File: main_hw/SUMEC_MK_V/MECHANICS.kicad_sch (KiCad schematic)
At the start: 16 parts, among them SW2 SW_Push, SW3 SW_Push, SW4 SW_Push, SW5 SW_Push

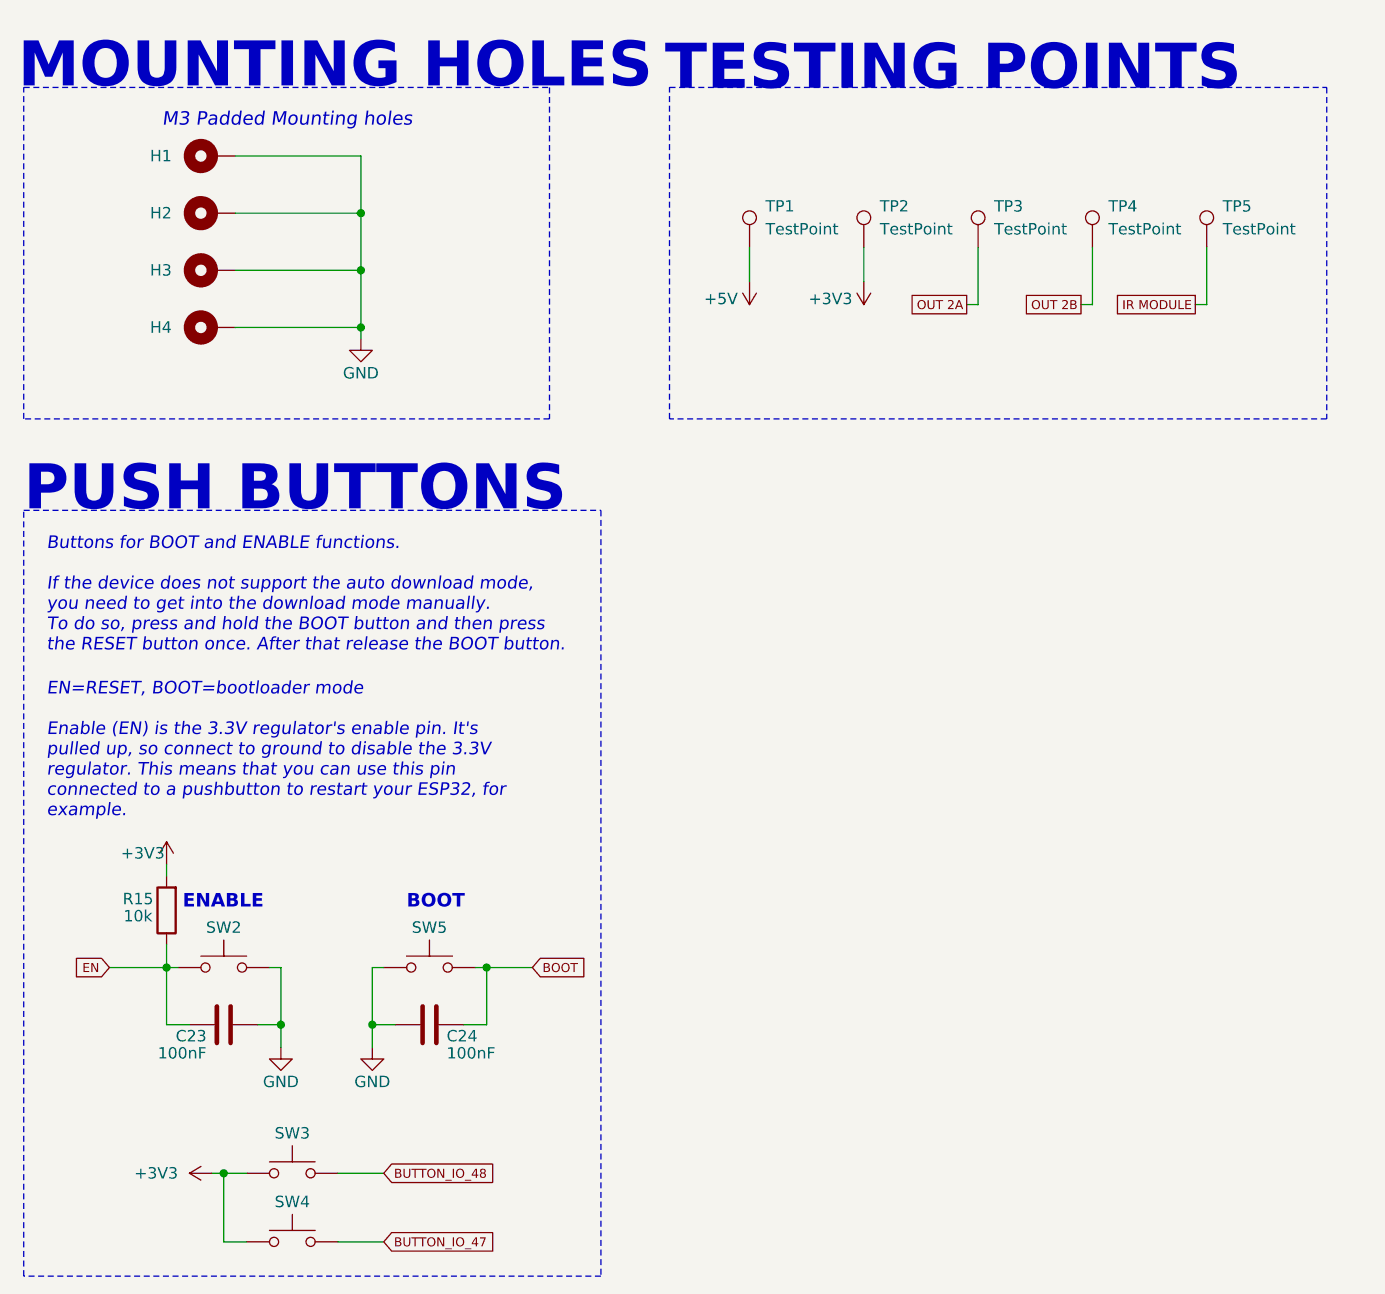
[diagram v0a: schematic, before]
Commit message: MK V Schematic update
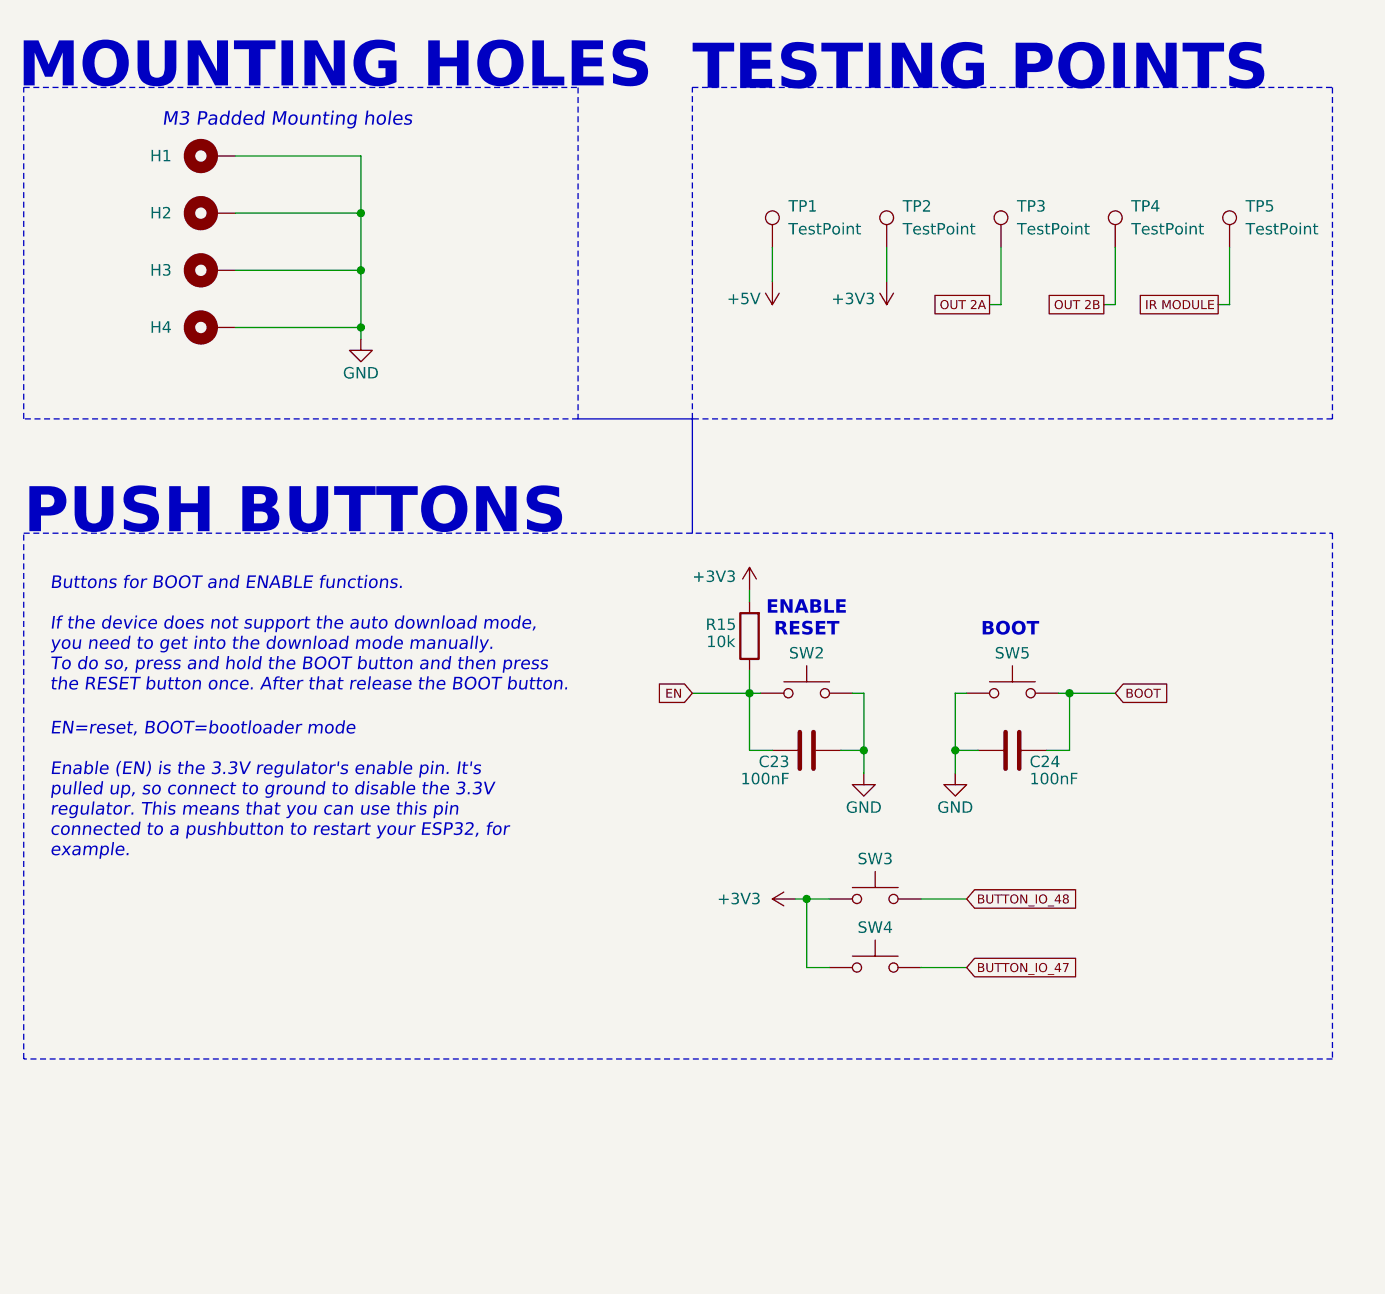
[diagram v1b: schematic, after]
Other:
- note added: "EN=reset, BOOT=bootloader mode Enable (EN) is the 3.3V regulator's enable pin. It's pulled up, so connect to ground to disable the 3.3V regulator. This means that you can use this pin connected to a pushbutton to restart your ESP32, for example."
- note added: "ENABLE RESET"
- note removed: "EN=RESET, BOOT=bootloader mode Enable (EN) is the 3.3V regulator's enable pin. It's pulled up, so connect to ground to disable the 3.3V regulator. This means that you can use this pin connected to a pushbutton to restart your ESP32, for example."
- note removed: "ENABLE"
- moved on the sheet: C23, C24, R15, SW2, SW3, SW4, SW5, TP1, TP2, TP3, TP4, TP5
